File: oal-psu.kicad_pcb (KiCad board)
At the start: 2 copper layers, 200 x 80 mm, 61 parts, among them J1 MAINS_LINE, J2 MAINS_NEUTRAL, J3 OUTPUT, P101 ENABLE_A, P2 OUTPUT_SELECT, P201 ENABLE_B, SW1 DPDT_SLIDE, SW102 VOLTAGE_A, SW202 VOLTAGE_B, T1 TALEMA 15/25VA, U101 TPS7A4700, U201 TPS7A4700

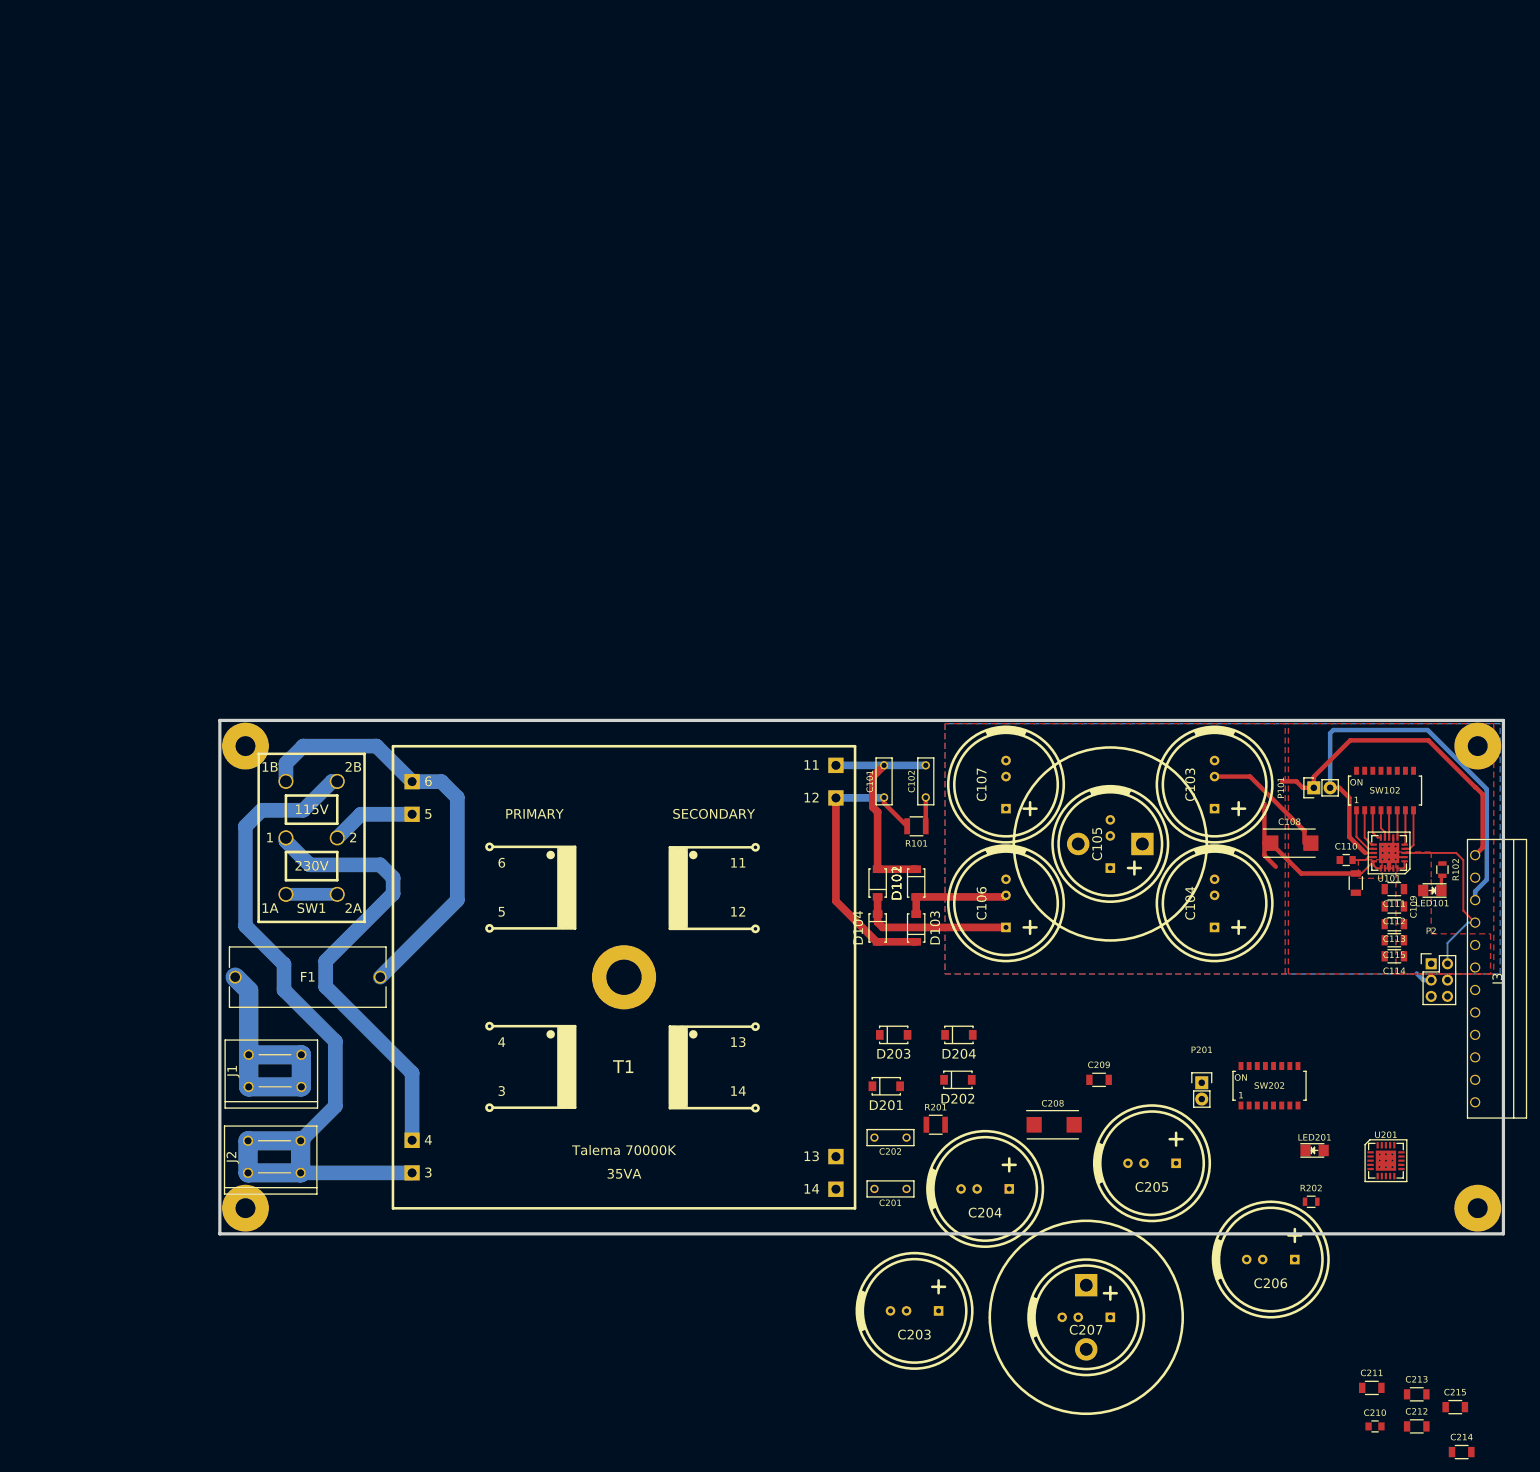
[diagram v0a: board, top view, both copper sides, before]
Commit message: finished initial layout
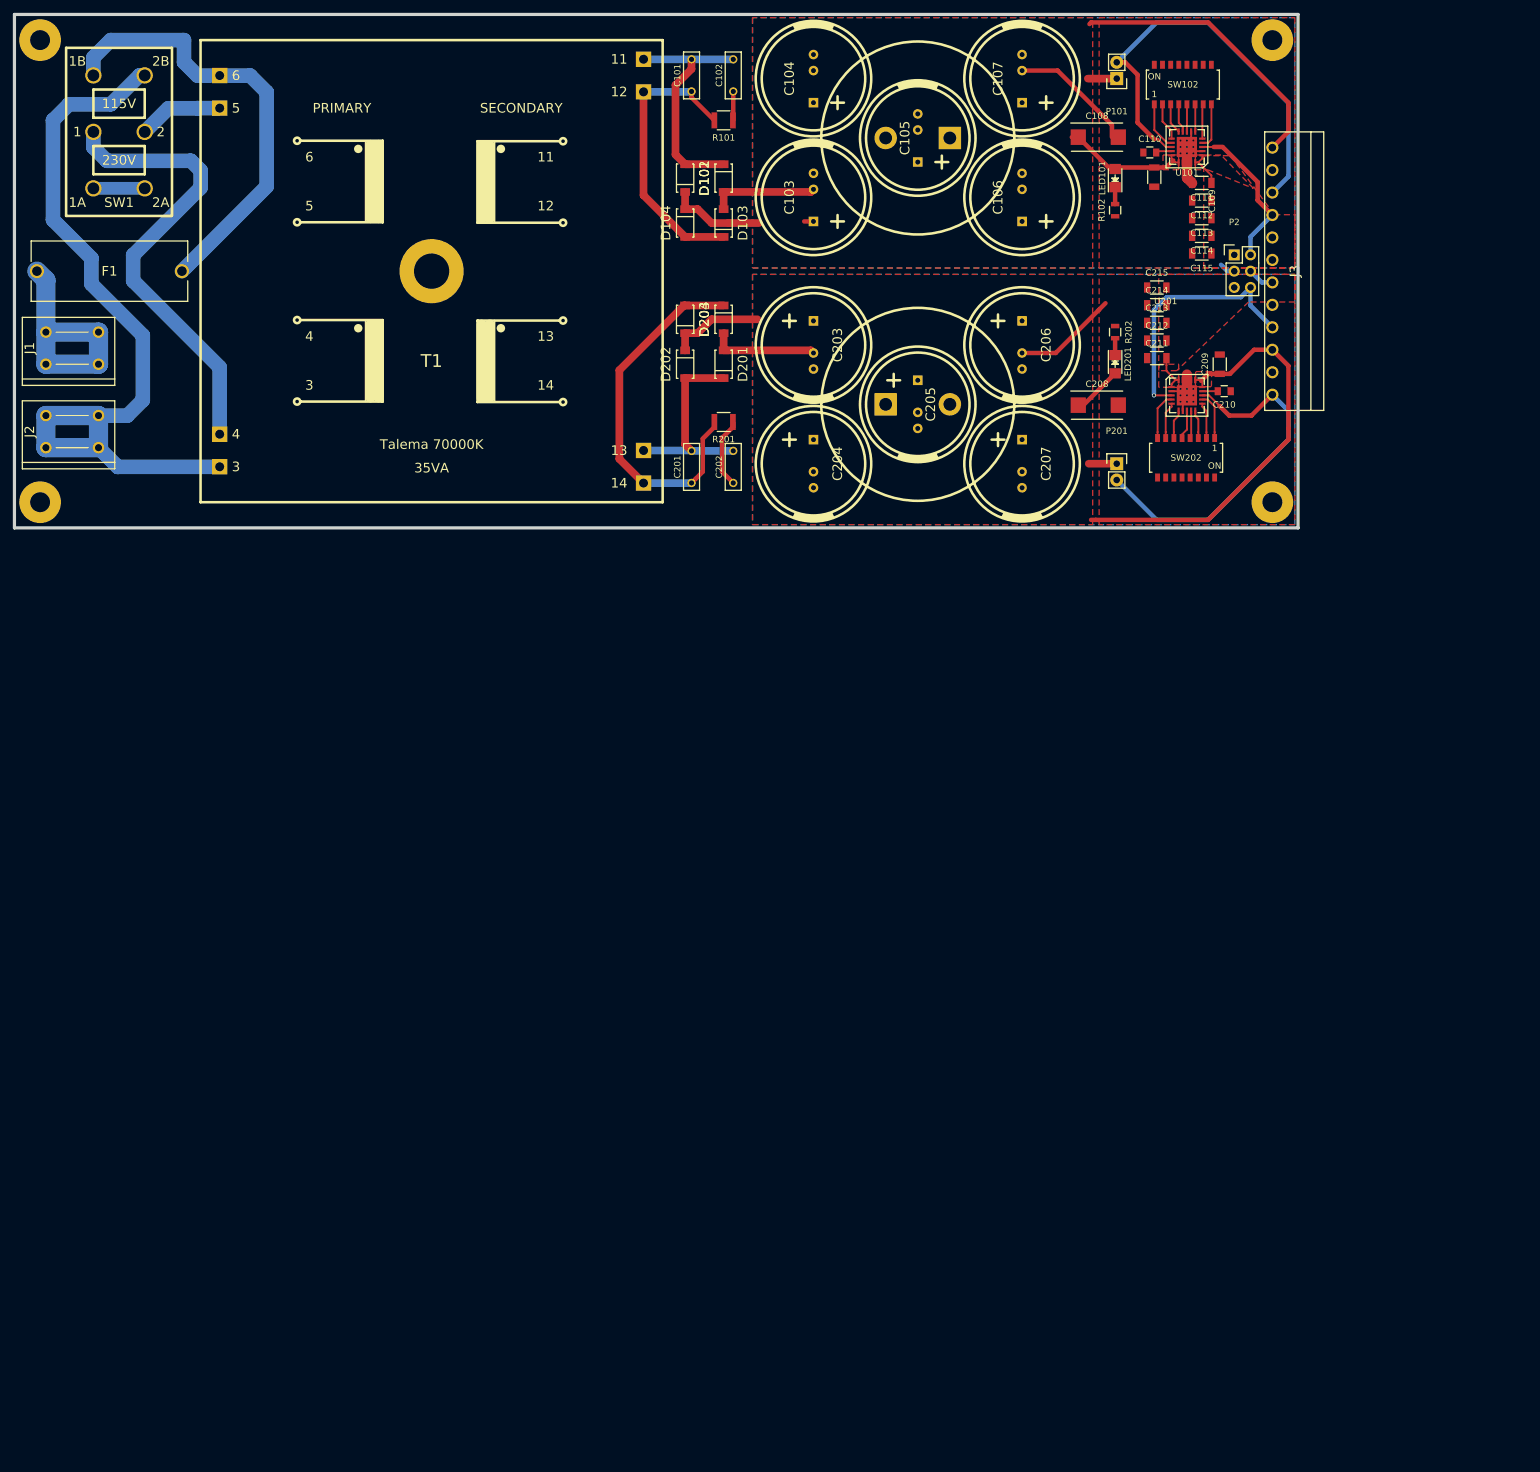
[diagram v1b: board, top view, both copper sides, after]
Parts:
- removed REF** (x4): MOUNTING_HOLE-M3, MOUNTING_HOLE-M3
- added X1: M3 HOLE, ose-audio-labs:MOUNTING_HOLE-M3, F.Cu at (4.00, 36.0)
- added X2: M3 HOLE, ose-audio-labs:MOUNTING_HOLE-M3, F.Cu at (4.00, -36.0)
- added X3: M3 HOLE, ose-audio-labs:MOUNTING_HOLE-M3, F.Cu at (196.0, -36.0)
- added X4: M3 HOLE, ose-audio-labs:MOUNTING_HOLE-M3, F.Cu at (196.0, 36.0)
- C205: footprint ose-audio-labs:35V-LYTIC-7.5-5 -> ose-audio-labs:35V-LYTIC-7.5-5-10snap
- C207: footprint ose-audio-labs:35V-LYTIC-7.5-5-10snap -> ose-audio-labs:35V-LYTIC-7.5-5
- F1: footprint ose-audio-labs:LITTLEFUSE-0PTF0078P -> LITTLEFUSE-0PTF0078P
- J1: footprint ose-audio-labs:PHEONIX_SPT_5-2POS -> PHEONIX_SPT_5-2POS
- SW1: footprint ose-audio-labs:CK_V80212MS02Q-VOLTAGE_SELECTOR -> CK_V80212MS02Q-VOLTAGE_SELECTOR
- U101: footprint PVQFN-N20-new -> PVQFN-N20
- moved C214 184.9 mm to (178.0, 5.30)
- moved C215 180.5 mm to (178.0, 2.55)
- moved C212 174.0 mm to (178.0, 10.8)
- moved C213 171.8 mm to (178.0, 8.05)
- moved C211 163.9 mm to (178.0, 13.6)
- moved C210 163.0 mm to (188.5, 18.7), turned to 180 degrees
- moved C203 151.3 mm to (124.5, 11.5), turned to 90 degrees
- moved C206 147.7 mm to (157.0, 11.5), turned to 90 degrees
- moved C104 142.9 mm to (124.5, -30.0)
- moved R202 138.9 mm to (171.5, 9.50), turned to 270 degrees
- moved C207 133.4 mm to (157.0, 30.0), turned to 90 degrees
- moved LED201 126.4 mm to (171.5, 14.5), turned to 270 degrees
- moved C205 123.8 mm to (140.8, 20.8), turned to 90 degrees
- moved U201 123.2 mm to (182.7, 19.4)
- moved LED101 121.5 mm to (171.5, -14.5), turned to 90 degrees
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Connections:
- J3 pad 1: UNREG-B -> ENABLE-B
- J3 pad 3: ENABLE-B -> UNREG-B
- LED101 pad 2: POS-A -> UNREG-A
- LED201 pad 2: POS-B -> UNREG-B
- U201 pad 10: Net-(SW202-Pad6) -> Net-(SW202-Pad3)
- U201 pad 11: Net-(SW202-Pad7) -> Net-(SW202-Pad2)
- U201 pad 12: Net-(SW202-Pad8) -> Net-(SW202-Pad1)
- U201 pad 4: Net-(SW202-Pad1) -> Net-(SW202-Pad8)
- U201 pad 5: Net-(SW202-Pad2) -> Net-(SW202-Pad7)
- U201 pad 6: Net-(SW202-Pad3) -> Net-(SW202-Pad6)
- U201 pad 8: Net-(SW202-Pad4) -> Net-(SW202-Pad5)
- U201 pad 9: Net-(SW202-Pad5) -> Net-(SW202-Pad4)
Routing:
- net UNREG-B: track 0.00 -> 93.7 mm
- net Net-(C201-Pad2): track 0.00 -> 58.0 mm
- net ENABLE-B: track 0.00 -> 56.1 mm
- net NEG-B: track 0.00 -> 41.9 mm
- net SENSE-B: track 0.00 -> 40.2 mm, vias 0 -> 1
- net Net-(C201-Pad1): track 0.00 -> 31.8 mm
- net UNREG-A: track 106.2 -> 84.6 mm
- net Net-(C202-Pad2): track 0.00 -> 10.9 mm
- net POS-B: track 0.00 -> 9.94 mm
- net NEG-A: track 44.7 -> 54.1 mm
- net Net-(SW202-Pad8): track 0.00 -> 7.37 mm
- net Net-(SW202-Pad1): track 0.00 -> 7.29 mm
- net Net-(SW202-Pad7): track 0.00 -> 5.73 mm
- net Net-(SW202-Pad2): track 0.00 -> 5.62 mm
- net Net-(SW202-Pad5): track 0.00 -> 4.57 mm
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- added copper zone on B.Cu, net NEG-B
- added copper zone on F.Cu, net NEG-B
- added copper zone on F.Cu, net POS-B
- added copper zone on F.Cu, net UNREG-B
